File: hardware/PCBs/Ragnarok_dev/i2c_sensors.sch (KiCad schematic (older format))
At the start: 9 parts, among them U10 SDP32, U9 BNO055

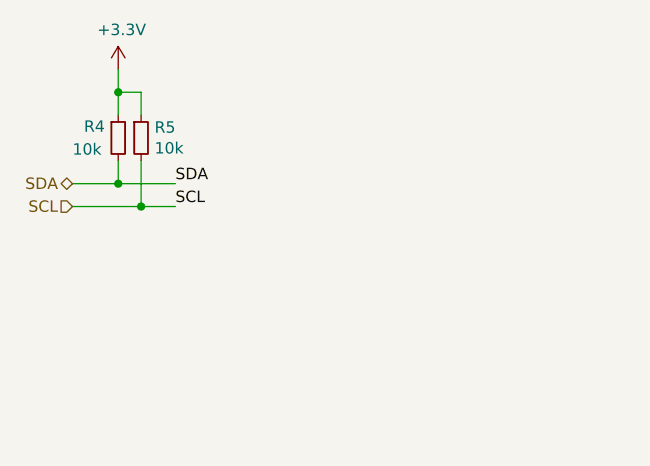
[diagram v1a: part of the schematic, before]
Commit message: update
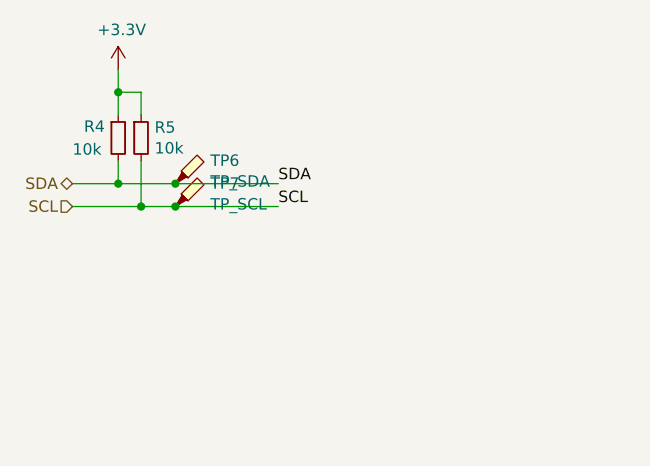
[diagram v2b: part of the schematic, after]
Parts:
- added TP6: TP_SDA, TestPoint:TestPoint_Pad_1.0x1.0mm, symbol Connector:TestPoint_Probe
- added TP7: TP_SCL, TestPoint:TestPoint_Pad_1.0x1.0mm, symbol Connector:TestPoint_Probe
- C30, C31, C32, C33, C34: footprint (none) -> Capacitor_SMD:C_0603_1608Metric_Pad1.05x0.95mm_HandSolder
- R4, R5: footprint (none) -> Resistor_SMD:R_0603_1608Metric_Pad1.05x0.95mm_HandSolder
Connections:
- net SCL: now also TP7.1
- net SDA: now also TP6.1
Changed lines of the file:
@@
 Text HLabel 900  1350 0    50   Input ~ 0
 SCL
-Text Label 1350 1250 0    50   ~ 0
+Text Label 1800 1250 0    50   ~ 0
 SDA
-Text Label 1350 1350 0    50   ~ 0
+Text Label 1800 1350 0    50   ~ 0
 SCL
 $Comp
@@
 F 0 "R4" H 950 1100 50  0000 L CNN
 F 1 "10k" H 900 1000 50  0000 L CNN
-F 2 "" H 1100 1050 50  0001 C CNN
+F 2 "Resistor_SMD:R_0603_1608Metric_Pad1.05x0.95mm_HandSolder" H 1100 1050 50  0001 C CNN
 F 3 "~" H 1100 1050 50  0001 C CNN
 	1    1100 1050
@@
 F 0 "R5" H 1259 1096 50  0000 L CNN
 F 1 "10k" H 1259 1005 50  0000 L CNN
-F 2 "" H 1200 1050 50  0001 C CNN
+F 2 "Resistor_SMD:R_0603_1608Metric_Pad1.05x0.95mm_HandSolder" H 1200 1050 50  0001 C CNN
 F 3 "~" H 1200 1050 50  0001 C CNN
 	1    1200 1050
@@
 F 0 "C33" H 6092 5446 50  0000 L CNN
 F 1 "0.1uF" H 6092 5355 50  0000 L CNN
-F 2 "" H 6000 5400 50  0001 C CNN
+F 2 "Capacitor_SMD:C_0603_1608Metric_Pad1.05x0.95mm_HandSolder" H 6000 5400 50  0001 C CNN
 F 3 "~" H 6000 5400 50  0001 C CNN
 	1    6000 5400
@@
 F 0 "C30" V 4821 1950 50  0000 C CNN
 F 1 "0.1uF" V 4912 1950 50  0000 C CNN
-F 2 "" H 5050 1950 50  0001 C CNN
+F 2 "Capacitor_SMD:C_0603_1608Metric_Pad1.05x0.95mm_HandSolder" H 5050 1950 50  0001 C CNN
 F 3 "~" H 5050 1950 50  0001 C CNN
 	1    5050 1950
@@
 F 0 "C34" V 5871 3350 50  0000 C CNN
 F 1 "0.1uF" V 5962 3350 50  0000 C CNN
-F 2 "" H 6100 3350 50  0001 C CNN
+F 2 "Capacitor_SMD:C_0603_1608Metric_Pad1.05x0.95mm_HandSolder" H 6100 3350 50  0001 C CNN
 F 3 "~" H 6100 3350 50  0001 C CNN
 	1    6100 3350
@@
 F 0 "C32" V 5250 1950 50  0000 C CNN
 F 1 "6.8nF" V 5350 1950 50  0000 C CNN
-F 2 "" H 5450 1950 50  0001 C CNN
+F 2 "Capacitor_SMD:C_0603_1608Metric_Pad1.05x0.95mm_HandSolder" H 5450 1950 50  0001 C CNN
 F 3 "~" H 5450 1950 50  0001 C CNN
 	1    5450 1950
@@
 F 0 "C31" V 5221 1600 50  0000 C CNN
 F 1 "120nF" V 5312 1600 50  0000 C CNN
-F 2 "" H 5450 1600 50  0001 C CNN
+F 2 "Capacitor_SMD:C_0603_1608Metric_Pad1.05x0.95mm_HandSolder" H 5450 1600 50  0001 C CNN
 F 3 "~" H 5450 1600 50  0001 C CNN
 	1    5450 1600
@@
 Text Notes 4700 5950 0    50   ~ 0
 Addr: 0x21\n
+$Comp
+L Connector:TestPoint_Probe TP?
+U 1 1 5E845BF0
+P 1350 1350
+AR Path="/5E845BF0" Ref="TP?"  Part="1"
+AR Path="/5E201923/5E845BF0" Ref="TP7"  Part="1"
+F 0 "TP7" H 1503 1451 50  0000 L CNN
+F 1 "TP_SCL" H 1503 1360 50  0000 L CNN
+F 2 "TestPoint:TestPoint_Pad_1.0x1.0mm" H 1550 1350 50  0001 C CNN
+F 3 "~" H 1550 1350 50  0001 C CNN
+	1    1350 1350
+	1    0    0    -1
+$EndComp
+$Comp
+L Connector:TestPoint_Probe TP?
+U 1 1 5E845BF6
+P 1350 1250
+AR Path="/5E845BF6" Ref="TP?"  Part="1"
+AR Path="/5E201923/5E845BF6" Ref="TP6"  Part="1"
+F 0 "TP6" H 1503 1351 50  0000 L CNN
+F 1 "TP_SDA" H 1503 1260 50  0000 L CNN
+F 2 "TestPoint:TestPoint_Pad_1.0x1.0mm" H 1550 1250 50  0001 C CNN
+F 3 "~" H 1550 1250 50  0001 C CNN
+	1    1350 1250
+	1    0    0    -1
+$EndComp
+Wire Wire Line
+	1350 1250 1800 1250
+Connection ~ 1350 1250
+Wire Wire Line
+	1350 1350 1800 1350
+Connection ~ 1350 1350
 $EndSCHEMATC
